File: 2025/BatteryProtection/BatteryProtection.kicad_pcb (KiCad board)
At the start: 4 copper layers, 90.9 x 36.6 mm, 43 parts, among them Q1 IXTA140P05T, Q10 BC849, Q11 BC849, Q2 BC849, Q3 BC849, Q4 BC849, Q5 BC849, Q6 BC849, Q7 BC849, Q8 BC849, Q9 BC849, U1 PLACEHOLDER, U2 PLACEHOLDER

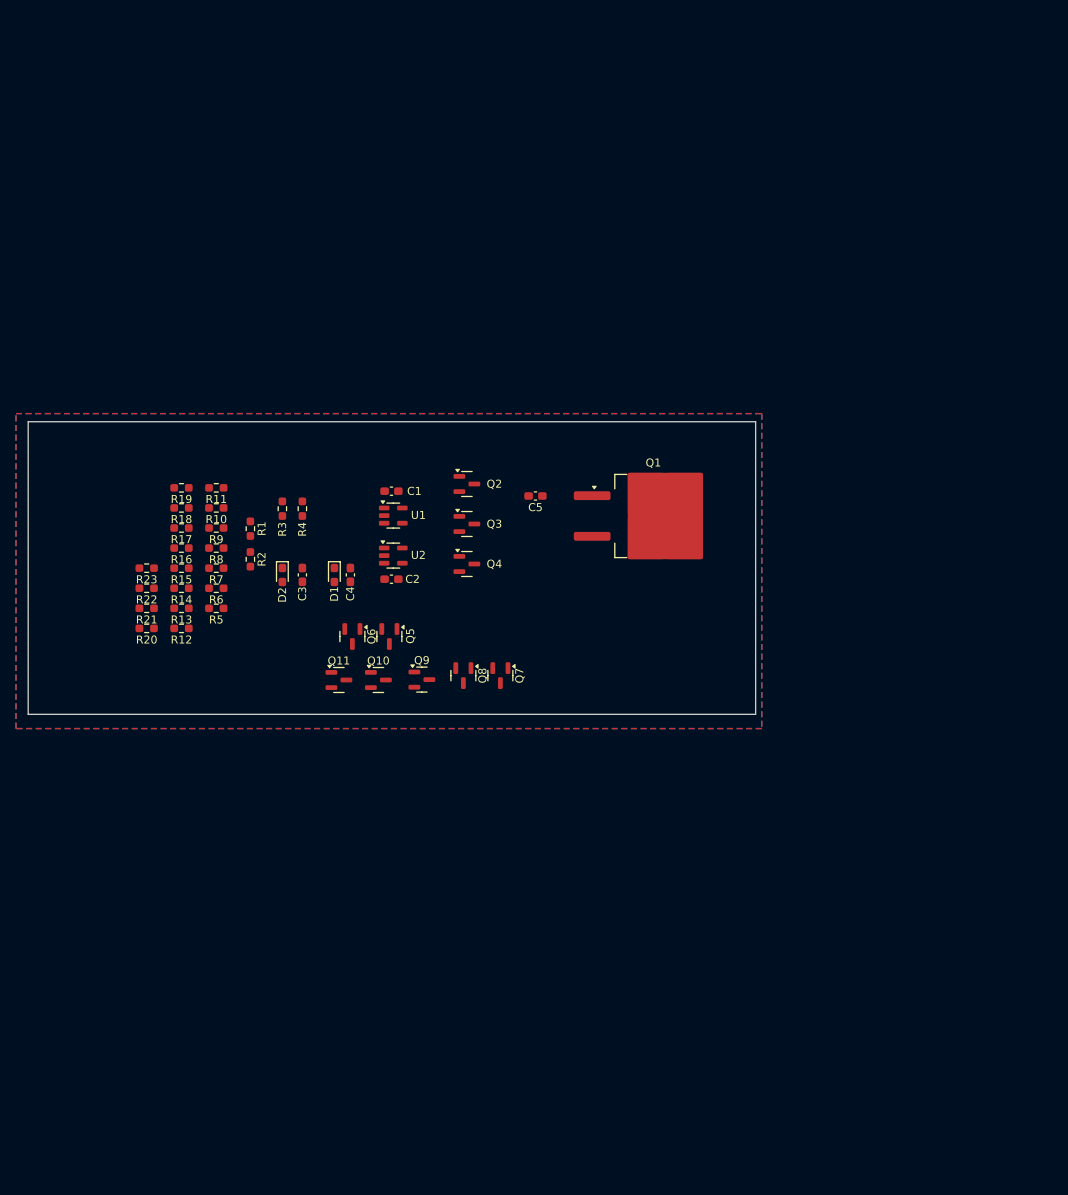
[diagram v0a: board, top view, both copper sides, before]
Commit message: started PCB layout
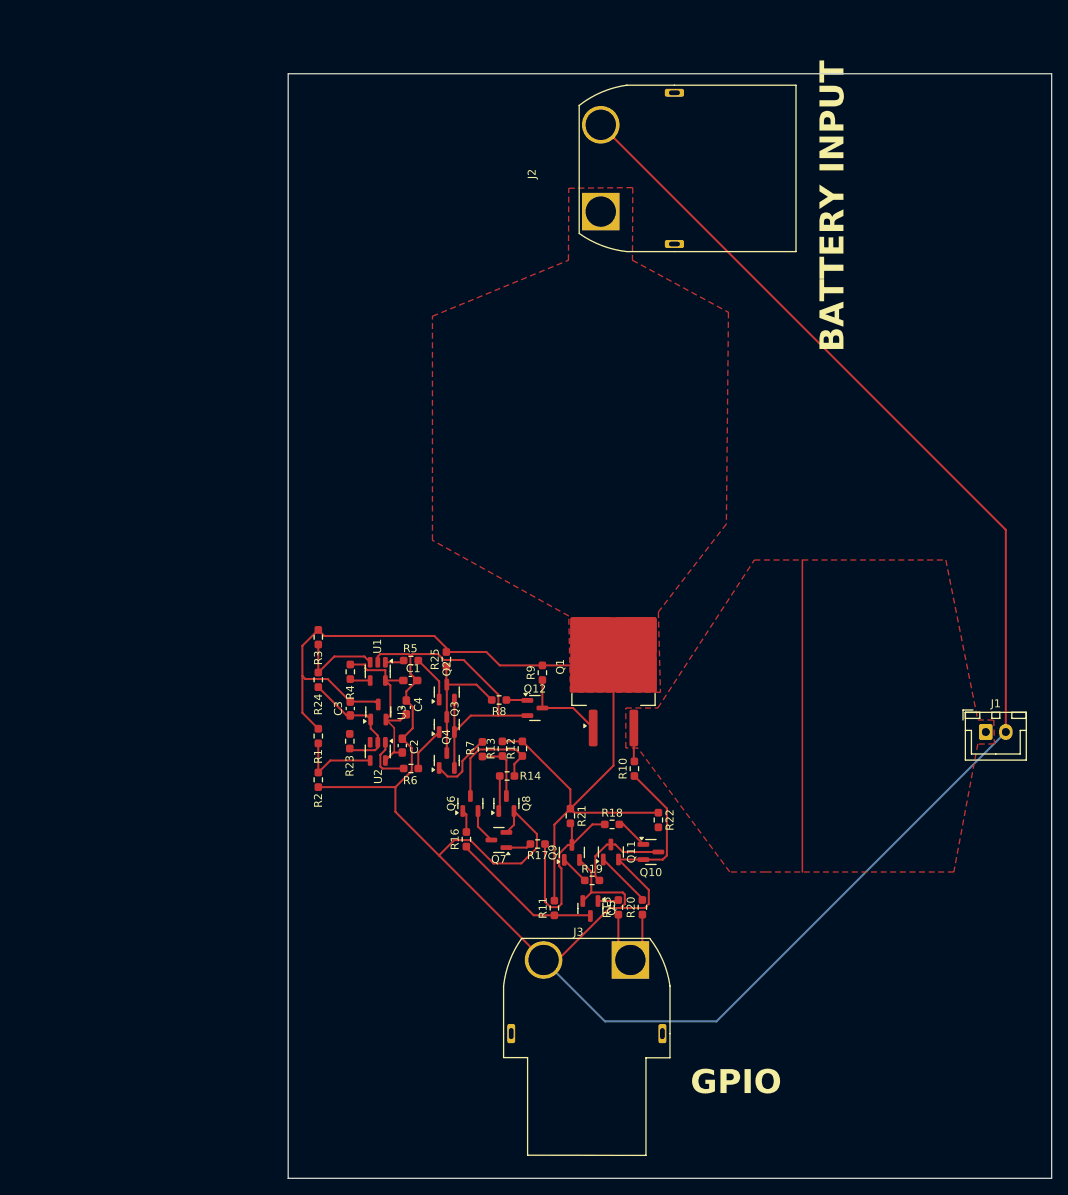
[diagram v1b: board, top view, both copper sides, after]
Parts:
- removed C5: 0.1uF, Capacitor_SMD:C_0603_1608Metric_Pad1.08x0.95mm_HandSolder
- removed D1: 4.7V, Diode_SMD:D_0603_1608Metric_Pad1.05x0.95mm_HandSolder
- removed D2: 5.6V, Diode_SMD:D_0603_1608Metric_Pad1.05x0.95mm_HandSolder
- added J1: Conn_01x02_Socket, Connector_JST:JST_XH_B2B-XH-A_1x02_P2.50mm_Vertical, F.Cu at (213.4, 116.0)
- added J2: Conn_01x02_Pin, BatteryProtection:XT90PW-M, F.Cu at (174.5, 46.0)
- added J3: Conn_01x02_Pin, BatteryProtection:XT90PW-F, F.Cu at (163.2, 153.7)
- added Q12: BC847, Package_TO_SOT_SMD:SOT-23, F.Cu at (157.1, 113.0)
- added R24: 10k, Resistor_SMD:R_0603_1608Metric_Pad0.98x0.95mm_HandSolder, F.Cu at (130.0, 109.5)
- added R25: 100k, Resistor_SMD:R_0603_1608Metric_Pad0.98x0.95mm_HandSolder, F.Cu at (146.0, 106.9)
- added U3: MCP1799x-330xxTT, Package_TO_SOT_SMD:SOT-23, F.Cu at (137.5, 113.5)
- C1, C2: value 10nF -> 1uF
- C3, C4: value 1uF -> 1u
- Q10, Q11, Q2, Q3, Q4, Q5, Q6, Q7, Q8, Q9: value BC849 -> BC847
- R1, R10: value 100k -> 50k
- R11: value Load -> 100k
- R14, R8: value 100k -> 1k
- R2: value 50k -> 10k
- R23: value 1k -> 10k
- R3: value 10k -> 116k
- R4: value 10k -> 15k
- R9: value 1k -> 100k
- U1, U2: value PLACEHOLDER -> MCP6561-OT
- moved R20 71.1 mm to (170.5, 137.9), turned to 90 degrees
- moved R19 71.0 mm to (164.2, 134.6), turned to 0 degrees
- moved R22 70.2 mm to (172.5, 127.0), turned to -90 degrees
- moved R15 69.1 mm to (167.5, 137.9), turned to 90 degrees
- moved R11 67.4 mm to (159.5, 138.0), turned to 90 degrees
- moved R18 66.8 mm to (166.7, 127.5), turned to 0 degrees
- moved R10 61.6 mm to (169.5, 120.6), turned to 90 degrees
- moved R17 59.5 mm to (157.4, 130.0)
- moved R21 59.0 mm to (161.5, 126.5), turned to -90 degrees
- moved R16 50.9 mm to (148.5, 129.4), turned to 90 degrees
- moved R14 47.0 mm to (153.6, 121.5)
- moved R12 45.2 mm to (155.5, 118.1), turned to 90 degrees
- moved R9 44.6 mm to (158.0, 108.6), turned to 90 degrees
- moved R13 43.8 mm to (153.0, 118.1), turned to 90 degrees
- moved Q5 42.3 mm to (164.0, 138.1)
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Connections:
- C1 pad 1: Net-(D2-K) -> GND
- C1 pad 2: GND -> +5V
- C2 pad 1: Net-(D1-K) -> GND
- C2 pad 2: GND -> +5V
- C3 pad 1: GND -> Vs
- C3 pad 2: Vs -> GND
- C4 pad 1: GND -> +5V
- C4 pad 2: Vs -> GND
- Q1 pad 3: Net-(Q1-S) -> VOUT
- Q2 pad 2: Net-(Q2-E) -> GND
- Q2 pad 3: Vs -> Net-(Q2-C)
- Q3 pad 2: Net-(Q2-E) -> GND
- Q3 pad 3: Vs -> Net-(Q2-C)
- Q4 pad 2: Net-(Q2-E) -> GND
- Q4 pad 3: Vs -> Net-(Q2-C)
- R1 pad 2: Net-(U1-+) -> Net-(U2--)
- R10 pad 1: Net-(Q1-G) -> GND
- R10 pad 2: Vs -> VOUT
- R11 pad 1: GND -> Net-(Q5-C)
- R11 pad 2: Net-(Q1-S) -> Vs
- R12 pad 1: Net-(Q5-C) -> Net-(Q6-C)
- R13 pad 1: Net-(Q6-C) -> Net-(Q8-C)
- R14 pad 1: Net-(Q8-C) -> Net-(Q6-C)
- R14 pad 2: Vs -> Net-(Q8-B)
- R15 pad 1: Net-(Q6-C) -> GPIO
- R15 pad 2: Net-(Q8-B) -> Net-(Q5-B)
- R16 pad 1: Net-(Q9-C) -> Net-(Q5-C)
- R16 pad 2: Net-(Q7-B) -> Net-(Q6-B)
- R17 pad 1: Net-(Q5-C) -> Net-(Q9-C)
- R17 pad 2: Net-(Q6-B) -> Net-(Q7-B)
- R18 pad 1: Gpio -> Net-(Q9-C)
- R18 pad 2: Net-(Q5-B) -> Net-(Q10-B)
- R19 pad 1: Net-(Q9-C) -> Net-(Q9-B)
- R19 pad 2: Net-(Q10-B) -> Net-(Q10-C)
- R2 pad 1: Net-(U1-+) -> Net-(U2--)
- R20 pad 1: Net-(Q9-B) -> GPIO
- R20 pad 2: Net-(Q10-C) -> Net-(Q11-B)
- R21 pad 1: Gpio -> Vs
- R21 pad 2: Net-(Q11-B) -> Net-(Q9-C)
- R22 pad 2: Net-(Q9-C) -> Net-(Q10-C)
- R23 pad 1: Vs -> Net-(U1--)
- R23 pad 2: Net-(Q10-C) -> GND
- R3 pad 2: Net-(D2-K) -> Net-(U1-+)
- R4 pad 1: Vs -> +5V
- R4 pad 2: Net-(D1-K) -> Net-(U1--)
- R8 pad 1: GND -> Net-(Q12-B)
- R8 pad 2: Net-(Q2-E) -> Net-(Q2-C)
- R9 pad 2: Net-(Q2-E) -> Vs
- U1 pad 1: Net-(D2-K) -> Net-(R5-Pad2)
- U1 pad 4: Net-(R5-Pad2) -> Net-(U1--)
- U1 pad 5: Vs -> +5V
- U2 pad 1: Net-(U1-+) -> Net-(R6-Pad1)
- U2 pad 3: Net-(D1-K) -> Net-(U1--)
- U2 pad 4: Net-(R6-Pad1) -> Net-(U2--)
- U2 pad 5: Vs -> +5V
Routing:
- net GND: track 0.00 -> 363.8 mm
- net Vs: track 0.00 -> 123.0 mm
- net Net-(Q9-C): track 0.00 -> 26.1 mm
- net +5V: track 0.00 -> 25.7 mm
- net Net-(Q5-C): track 0.00 -> 19.2 mm
- net Net-(Q2-C): track 0.00 -> 17.2 mm
- net Net-(Q6-C): track 0.00 -> 14.9 mm
- net GPIO: track 0.00 -> 12.6 mm
- net Net-(Q10-C): track 0.00 -> 12.1 mm
- net Net-(U1-+): track 0.00 -> 11.1 mm
- net Net-(Q1-G): track 0.00 -> 10.9 mm
- net Net-(U2--): track 0.00 -> 10.8 mm
- net Net-(Q4-B): track 0.00 -> 8.39 mm
- net Net-(Q8-C): track 0.00 -> 7.73 mm
- net Net-(Q11-B): track 0.00 -> 7.49 mm
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- added copper zone on F.Cu, net VOUT
- added copper zone on F.Cu, net Vs
- removed copper zone on B.Cu, net GND
- removed copper zone on F.Cu, net GND
- removed copper zone on In1.Cu, net GND
- removed copper zone on In2.Cu, net GND
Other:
- board size 90.9 x 36.6 mm -> 95.4 x 138.1 mm
- copper layers 4 -> 2
- board text added: "BATTERY INPUT"
- board text added: "GPIO"
